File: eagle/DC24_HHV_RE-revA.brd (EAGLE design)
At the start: 25.4 x 22.9 mm, 11 parts, among them U1 PIC12F1571

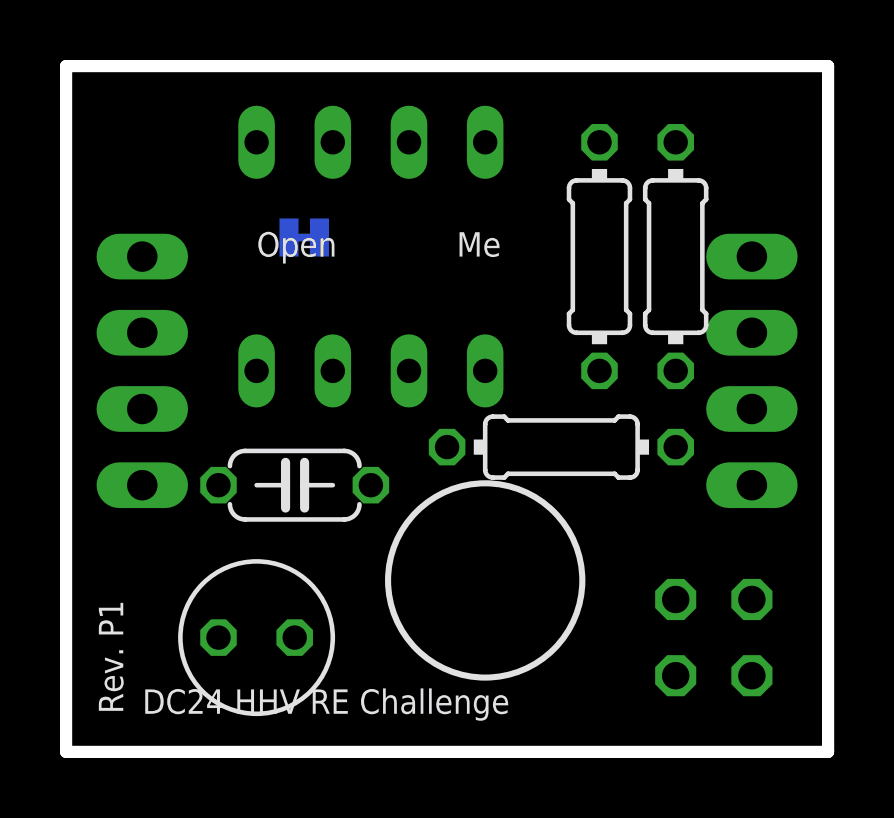
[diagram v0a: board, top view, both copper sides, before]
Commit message: Proposed final of rev A PCB Added CAM file and gerber files
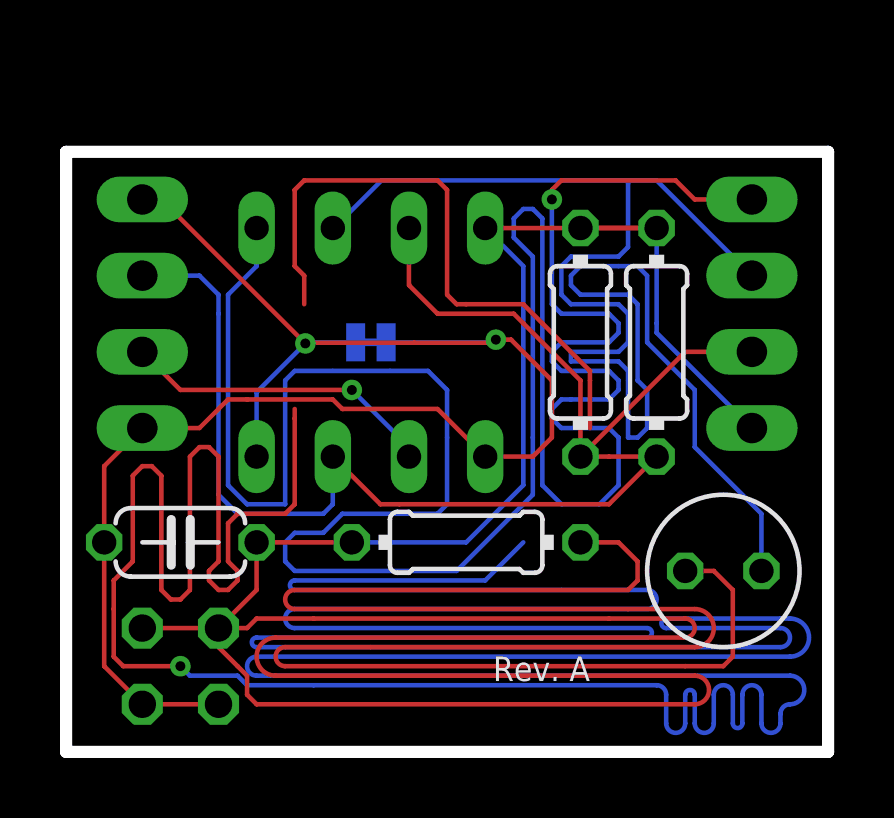
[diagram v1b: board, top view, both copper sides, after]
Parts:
- moved SV1 20.4 mm to (2.54, 14.6), turned to 270 degrees
- moved SV2 20.4 mm to (22.9, 14.6), turned to 90 degrees
- moved JP2 17.8 mm to (3.81, 2.86), turned to 180 degrees
- moved LED1 15.7 mm to (21.9, 6.03), turned to 0 degrees
- moved R1 4.49 mm to (13.3, 6.99), turned to 180 degrees
- moved C1 4.26 mm to (3.81, 6.99)
- moved JP3 4.14 mm to (10.2, 13.7), turned to 180 degrees
- moved R2 2.93 mm to (17.1, 13.7)
- moved R3 2.93 mm to (19.7, 13.7)
- moved U1 2.86 mm to (10.2, 13.7)
- moved U$1 2.86 mm to (5.71, 11.7)
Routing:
- net N$2: track 0.00 -> 185.0 mm, vias 0 -> 1
- net VCC: track 0.00 -> 104.8 mm
- net OTHER: track 0.00 -> 89.7 mm, vias 0 -> 1
- net N$3: track 0.00 -> 63.0 mm
- net LED: track 0.00 -> 53.7 mm
- net VSS: track 0.00 -> 38.7 mm, vias 0 -> 1
- net I2C_DAT: track 0.00 -> 29.6 mm
- net N$1: track 0.00 -> 20.5 mm
- net I2C_CLK: track 0.00 -> 18.6 mm
- net JUMPER: track 0.00 -> 17.2 mm, vias 0 -> 1
- net TX: track 0.00 -> 10.5 mm, vias 0 -> 1
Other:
- board size 25.4 x 22.9 mm -> 25.4 x 20 mm
- board text added: "+"
- board text added: "-"
- board text added: "CR2025"
- board text added: "Rev. A"
- board text removed: "Rev. P1"
